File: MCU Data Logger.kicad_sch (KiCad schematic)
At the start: 25 parts, among them U1 24LC1025, U2 24LC1025, U3 ATmega328P, U4 DS1337S_, Y1 Crystal, Y2 Crystal

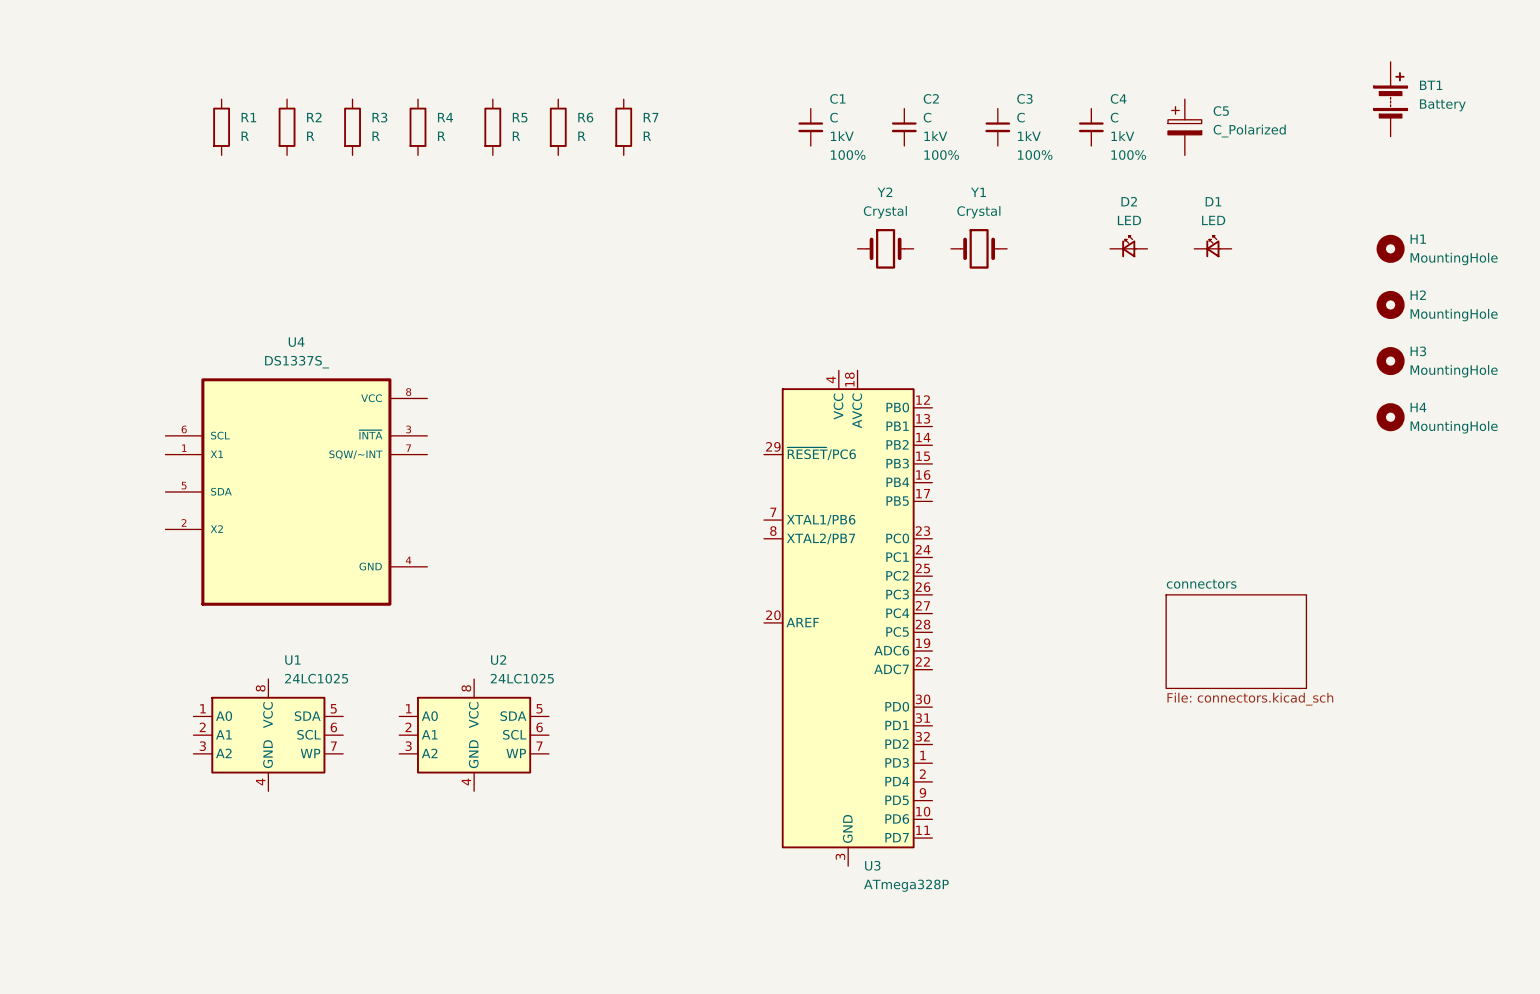
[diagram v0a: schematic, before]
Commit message: Editing some footprints
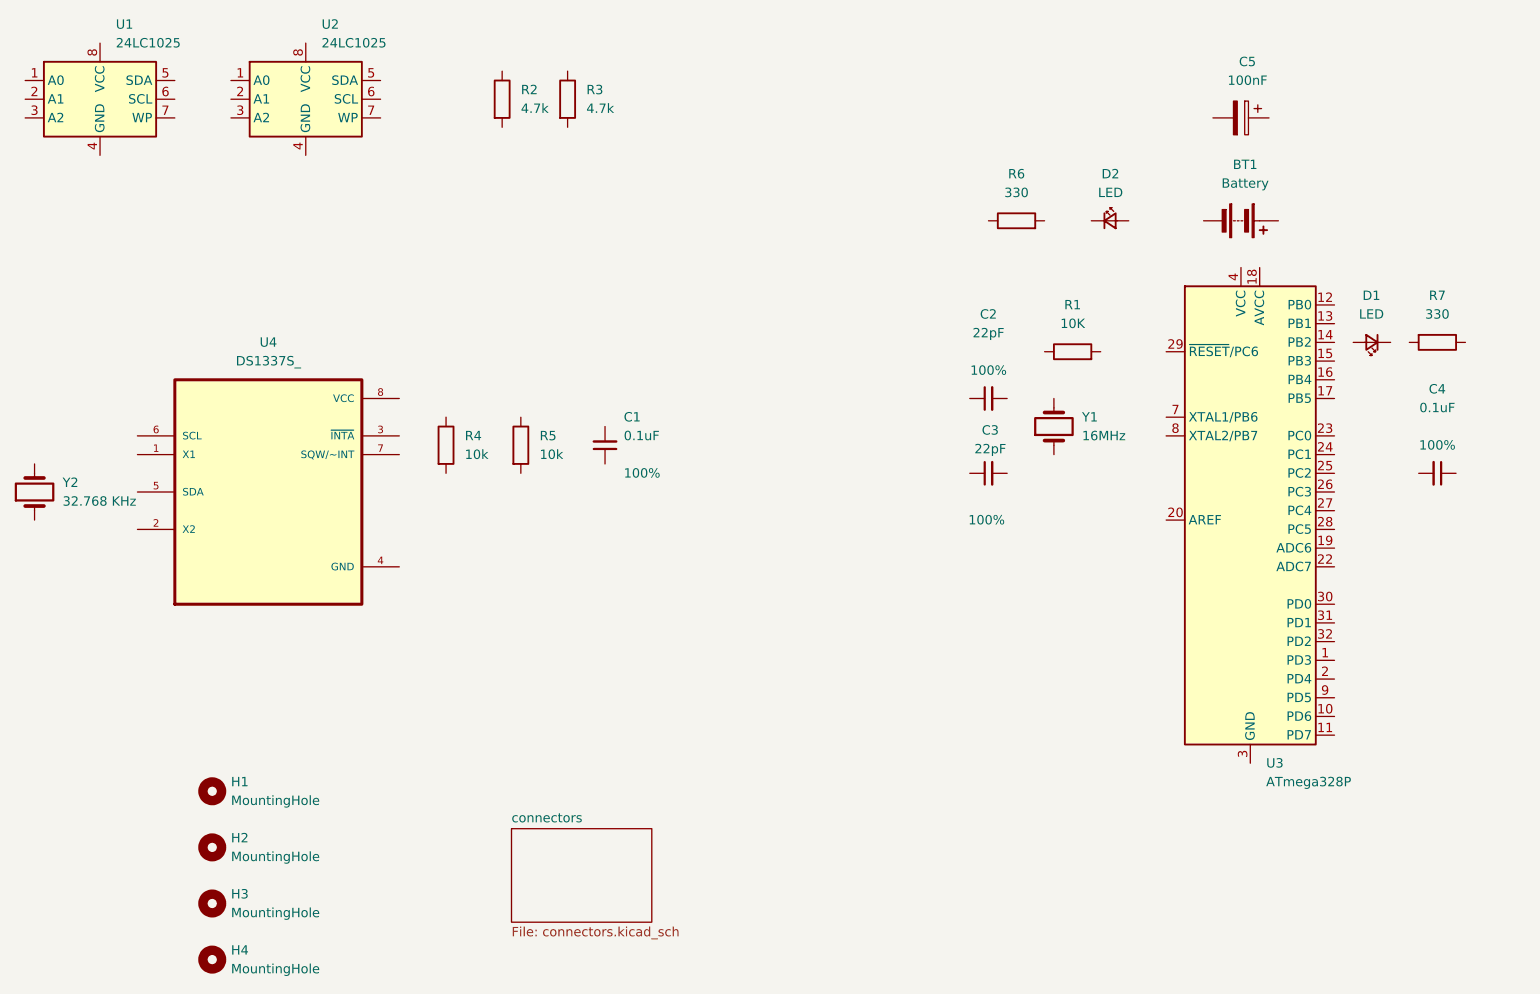
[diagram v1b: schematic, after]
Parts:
- BT1: footprint (none) -> TerminalBlock_Phoenix:TerminalBlock_Phoenix_MPT-0,5-2-2.54_1x02_P2.54mm_Horizontal
- C1, C4: value C -> 0.1uF; footprint SparkFun-Capacitor:C_0603_1608Metric -> Capacitor_SMD:C_0805_2012Metric
- C2, C3: value C -> 22pF; footprint SparkFun-Capacitor:C_0603_1608Metric -> Capacitor_SMD:C_0805_2012Metric
- C5: value C_Polarized -> 100nF; footprint (none) -> Capacitor_SMD:C_0805_2012Metric
- D1, D2: footprint SparkFun-LED:LED_0603_1608Metric -> LED_SMD:LED_0805_2012Metric
- H1, H2, H3, H4: footprint (none) -> MountingHole:MountingHole_2.1mm
- R1: value R -> 10K; footprint (none) -> Resistor_SMD:R_0805_2012Metric
- R2, R3: value R -> 4.7k; footprint (none) -> Resistor_SMD:R_0805_2012Metric
- R4, R5: value R -> 10k; footprint (none) -> Resistor_SMD:R_0805_2012Metric
- R6, R7: value R -> 330; footprint (none) -> Resistor_SMD:R_0805_2012Metric
- U1, U2: footprint (none) -> Package_SO:SOIC-8_3.9x4.9mm_P1.27mm
- U3: footprint SparkFun-Semiconductor-Standard:TQFP-32_7x7mm_P0.8mm -> footprints:QFP80P900X900X120-32N
- U4: footprint DS1337S_:SOIC127P600X175-8N -> footprints:SOIC127P600X175-8N
- Y1: value Crystal -> 16MHz; footprint (none) -> Crystal:Crystal_SMD_5032-2Pin_5.0x3.2mm_HandSoldering
- Y2: value Crystal -> 32.768 KHz; footprint (none) -> Crystal:Crystal_SMD_5032-2Pin_5.0x3.2mm_HandSoldering
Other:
- moved on the sheet: BT1, C1, C2, C3, C4, C5, D1, D2, H1, H2, H3, H4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
